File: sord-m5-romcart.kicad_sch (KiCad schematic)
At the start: 2 parts, among them U2 27C256

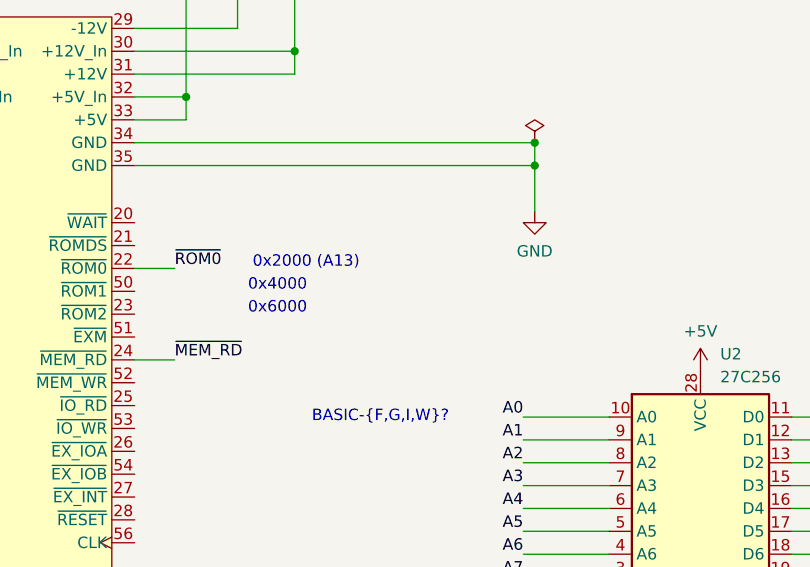
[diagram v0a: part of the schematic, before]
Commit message: Fumbling
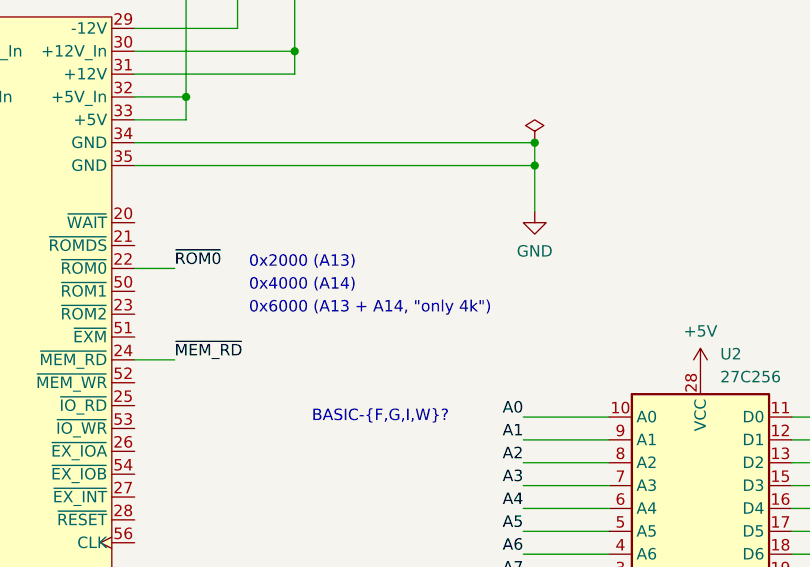
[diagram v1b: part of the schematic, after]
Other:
- note added: "0x4000 (A14)"
- note added: "0x6000 (A13 + A14, "only 4k")"
- note removed: "0x4000"
- note removed: "0x6000"
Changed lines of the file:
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@@
 	(text "0x2000 (A13)"
 		(exclude_from_sim no)
-		(at 122.555 67.31 0)
+		(at 116.205 67.31 0)
 		(effects
 			(font
 				(size 1.27 1.27)
 			)
+			(justify left)
 		)
 	)
-	(text "0x6000"
+	(text "0x6000 (A13 + A14, \"only 4k\")"
 		(exclude_from_sim no)
-		(at 119.38 72.39 0)
+		(at 116.205 72.39 0)
 		(effects
 			(font
 				(size 1.27 1.27)
 			)
+			(justify left)
 		)
 	)
@@
 		)
 	)
-	(text "0x4000"
+	(text "0x4000 (A14)"
 		(exclude_from_sim no)
-		(at 119.38 69.85 0)
+		(at 116.205 69.85 0)
 		(effects
 			(font
 				(size 1.27 1.27)
 			)
+			(justify left)
 		)
 	)
